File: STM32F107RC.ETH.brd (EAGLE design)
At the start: 160 x 100 mm, 43 parts, among them J1 HR911105A, J3 USB-MICROB, Q1 8MHz, U1 LAN8720A-CP, U2 STM32F107RCT6, U3 LM1117MP-3.3, X1 CB3LV-3I-74M2500, X2 MSTBA6

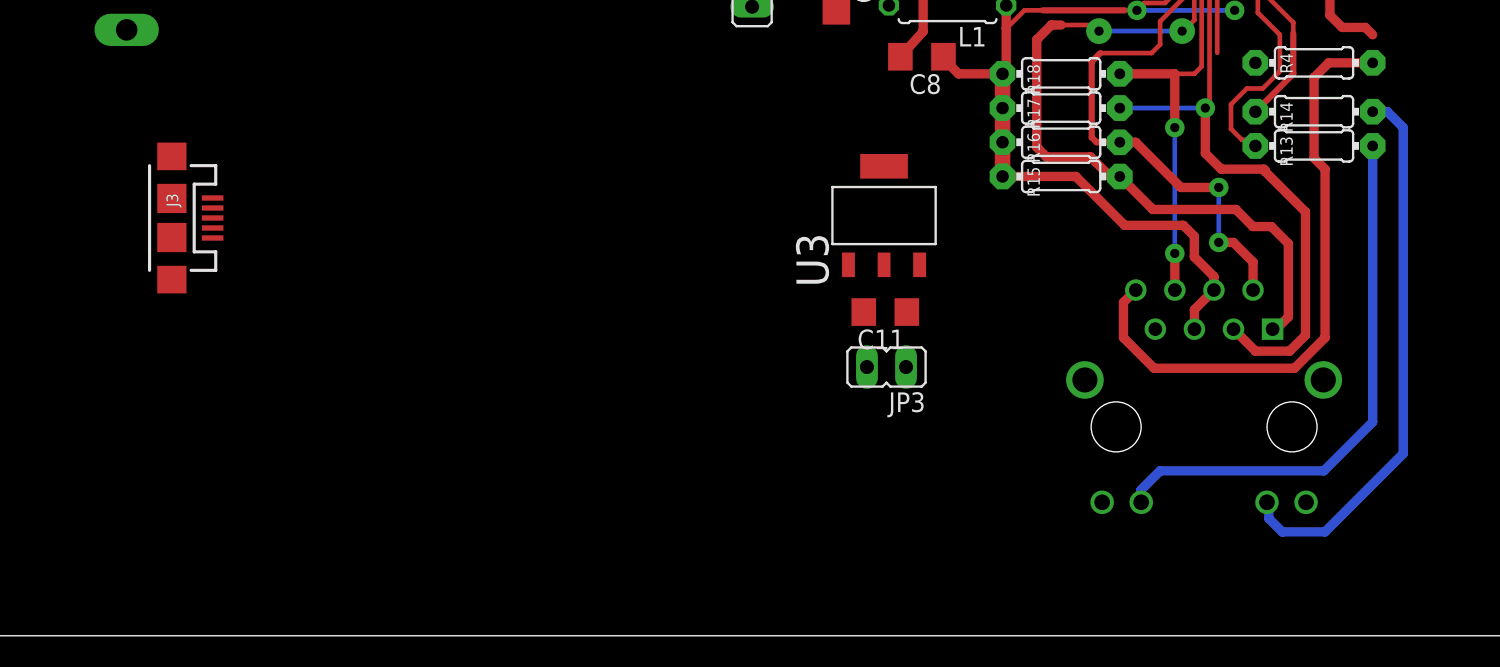
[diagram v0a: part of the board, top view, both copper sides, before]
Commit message: u 10-11-18
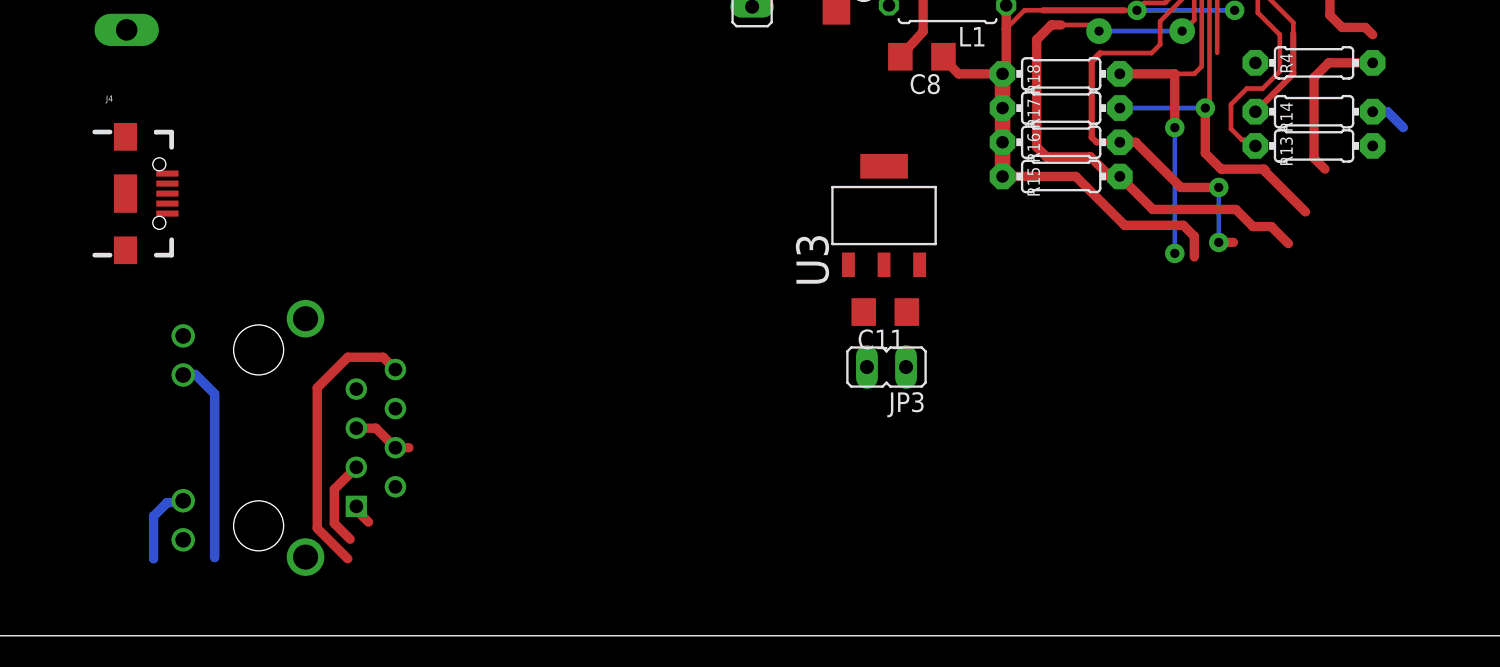
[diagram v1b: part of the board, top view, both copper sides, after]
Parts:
- removed J3: USB-MICROB, SparkFun-Connectors:USB-MICROB
- added J4: USB-MICROB", SparkFun-Connectors:USB-B-MICRO-SMD_V03
- moved J1 61.4 mm to (29.1, 12.9), turned to 270 degrees
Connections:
- net N$11 renamed SWO
- new net N$11: J4.D-, U2.44
- new net N$28: J4.D+, U2.45
- new net N$6: J4.VBUS, U2.42
- net GND: now also J4.GND
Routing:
- net LED1: track 35.9 -> 7.53 mm
- net LED2: track 35.7 -> 13.2 mm
- net GND: track 197.9 -> 187.0 mm
- net RD+: track 39.1 -> 31.1 mm
- net TD+: track 46.0 -> 41.3 mm
- net TD-: track 32.8 -> 29.2 mm
- net RD-: track 25.5 -> 23.2 mm
- net AVDD: track 56.9 -> 55.1 mm
